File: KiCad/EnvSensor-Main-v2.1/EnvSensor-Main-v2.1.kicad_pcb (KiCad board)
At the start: 4 copper layers, 102 x 100 mm, 92 parts, among them J1 Conn_01x02, J2 Conn_01x02, J3 HPMA115C0-003, J4 Conn_01x02, J5 Micro_SD_Card_Det, J6 SWD, J7 I2C, J8 POWER_INPUT, Q1 Si3407DV, Q2 IRLML2502, SW1 Reset, SW2 SW_Push, SW3 SW_Push, SW4 SW_Push, SW5 SW_Push, U1 BME280-Module, U2 BMP280, U3 SCD30, U4 SCD40, U5 STM32L451RCT6, U6 ESP-12S, U7 E-Ink_Waveshare_4.2, Y1 16MHz, Y2 32768/12.5pF

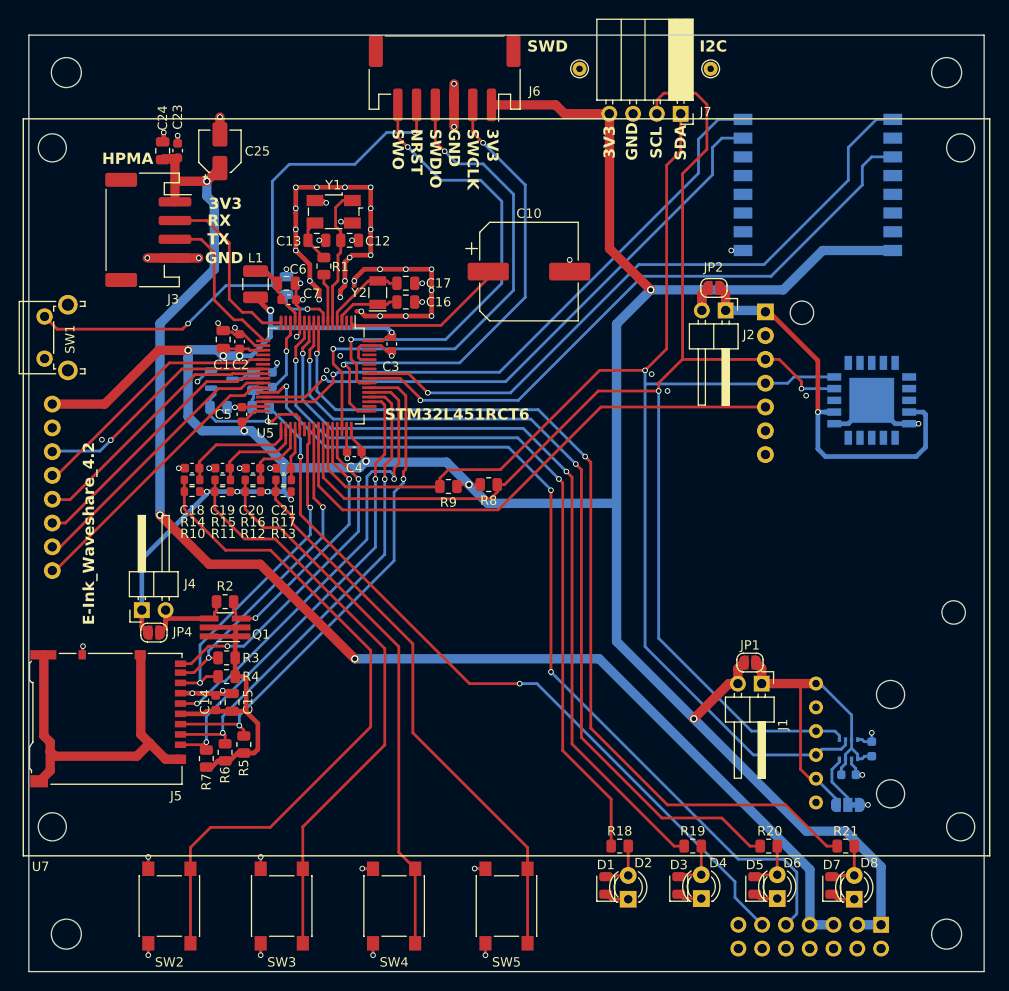
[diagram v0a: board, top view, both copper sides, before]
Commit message: Before moving i2c tracks
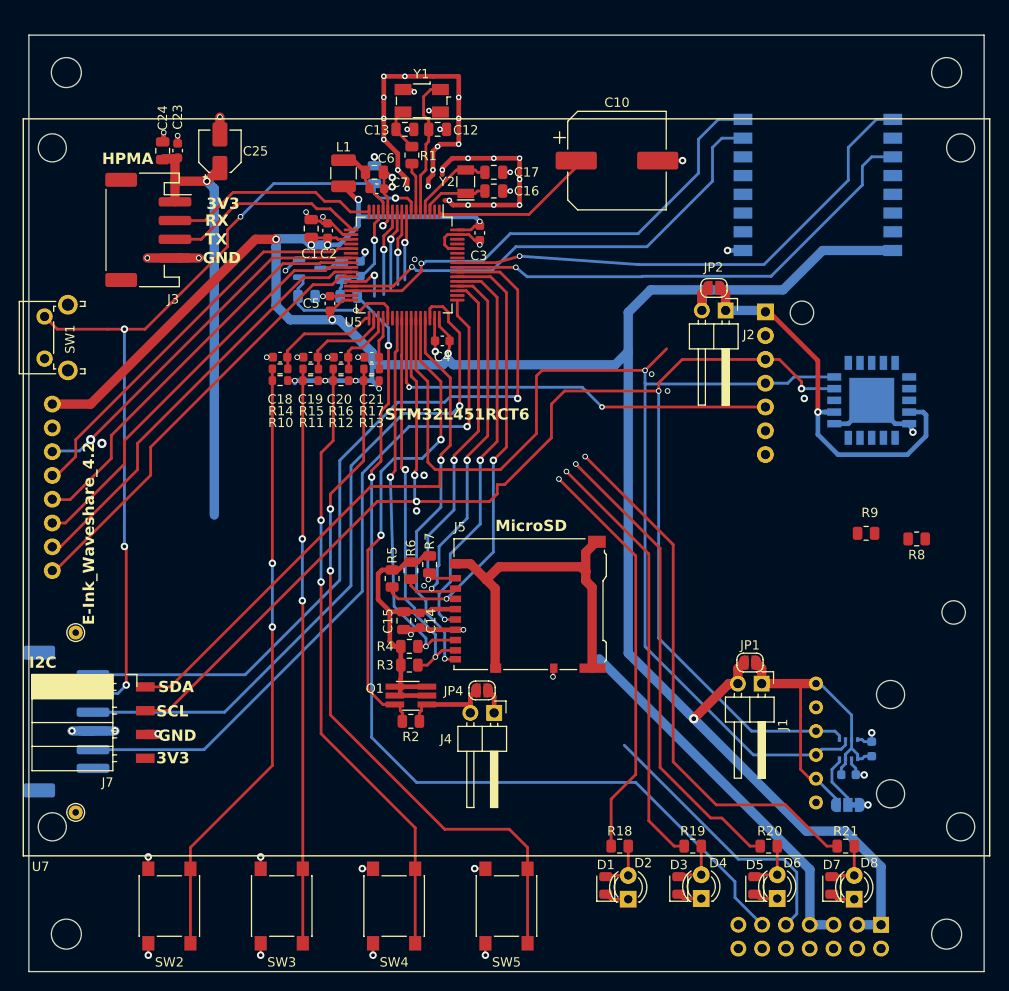
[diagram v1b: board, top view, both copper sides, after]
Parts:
- J6: moved to B.Cu
- J7: footprint Connector_PinSocket_2.54mm:PinSocket_1x04_P2.54mm_Horizontal -> JPConnectors:PinSocket_1x04_P2.54mm_Horizontal_SMD
- moved H5 95.9 mm to (25.0, 103.0), turned to 90 degrees
- moved H6 90.7 mm to (25.0, 83.8), turned to 90 degrees
- moved J7 85.1 mm to (30.4, 89.6), turned to 0 degrees
- moved J6 79.7 mm to (24.0, 93.3), turned to 90 degrees
- moved J5 46.4 mm to (73.3, 80.8), turned to 90 degrees
- moved R8 46.1 mm to (114.8, 73.8)
- moved R9 44.9 mm to (109.4, 73.2)
- moved J4 39.2 mm to (69.7, 92.4), turned to -90 degrees
- moved JP4 35.6 mm to (68.4, 90.0), turned to 180 degrees
- moved R7 31.6 mm to (62.8, 76.5), turned to 90 degrees
- moved R6 27.7 mm to (60.8, 77.2), turned to 90 degrees
- moved R5 23.8 mm to (58.8, 78.0), turned to 90 degrees
- moved R2 23.6 mm to (60.8, 93.3), turned to 180 degrees
- moved C14 23.6 mm to (61.8, 82.5), turned to 90 degrees
- moved Q1 21.1 mm to (60.8, 90.5), turned to 0 degrees
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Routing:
- net POWER_5V_ENABLE: track 98.6 -> 35.9 mm, vias 3 -> 1
- net +5V: track 143.4 -> 87.8 mm, vias 3 -> 1
- net +3V3: track 314.6 -> 268.1 mm, vias 14 -> 12
- net LED_4: track 99.7 -> 65.1 mm
- net LED_3: track 92.7 -> 58.2 mm
- net SWO: track 49.8 -> 84.1 mm, vias 2 -> 1
- net LED_2: track 85.6 -> 54.3 mm
- net LED_1: track 82.1 -> 52.9 mm
- net NRST: track 66.6 -> 91.7 mm, vias 3 -> 5
- net SWCLK: track 51.2 -> 75.7 mm, vias 2 -> 1
- net SDIO_POWER_ENABLE: track 29.1 -> 51.0 mm
- net SWDIO: track 54.7 -> 74.0 mm, vias 2 -> 1
- net SDA: track 150.9 -> 170.1 mm
- net +BATT: track 81.8 -> 100.7 mm
- net E_INK_BUSY: track 30.6 -> 46.7 mm
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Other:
- board text added: "MicroSD"
